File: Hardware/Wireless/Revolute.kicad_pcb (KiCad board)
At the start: 4 copper layers, 20 x 20 mm, 54 parts, among them Q1 AO3407, U1 BQ27441-G1, U2 nrf52833_qfn40, U3 AS5600, U4 AP2112K-3.3, U5 BQ24075RGT, U7 MAX16054, X1 32.768 kHz, X2 32MHZ

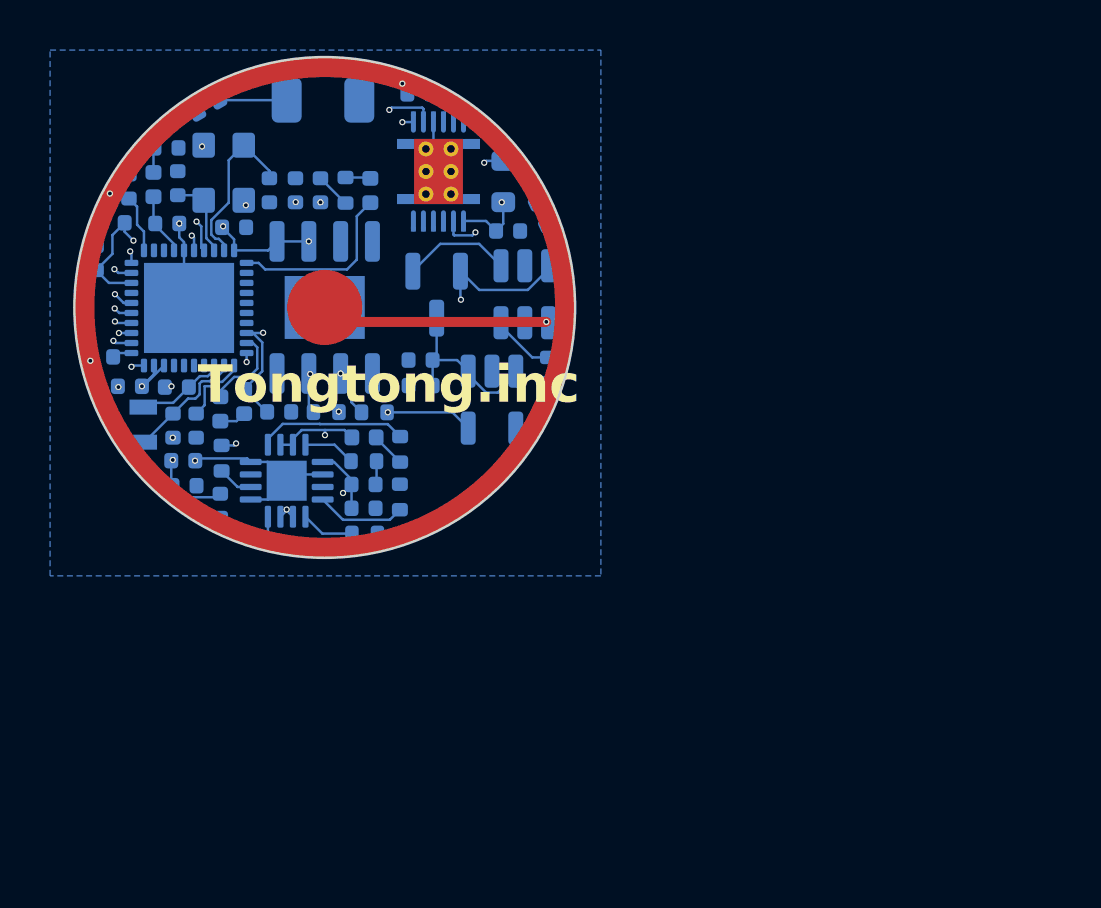
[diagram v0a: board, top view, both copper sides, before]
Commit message: worked on wireless
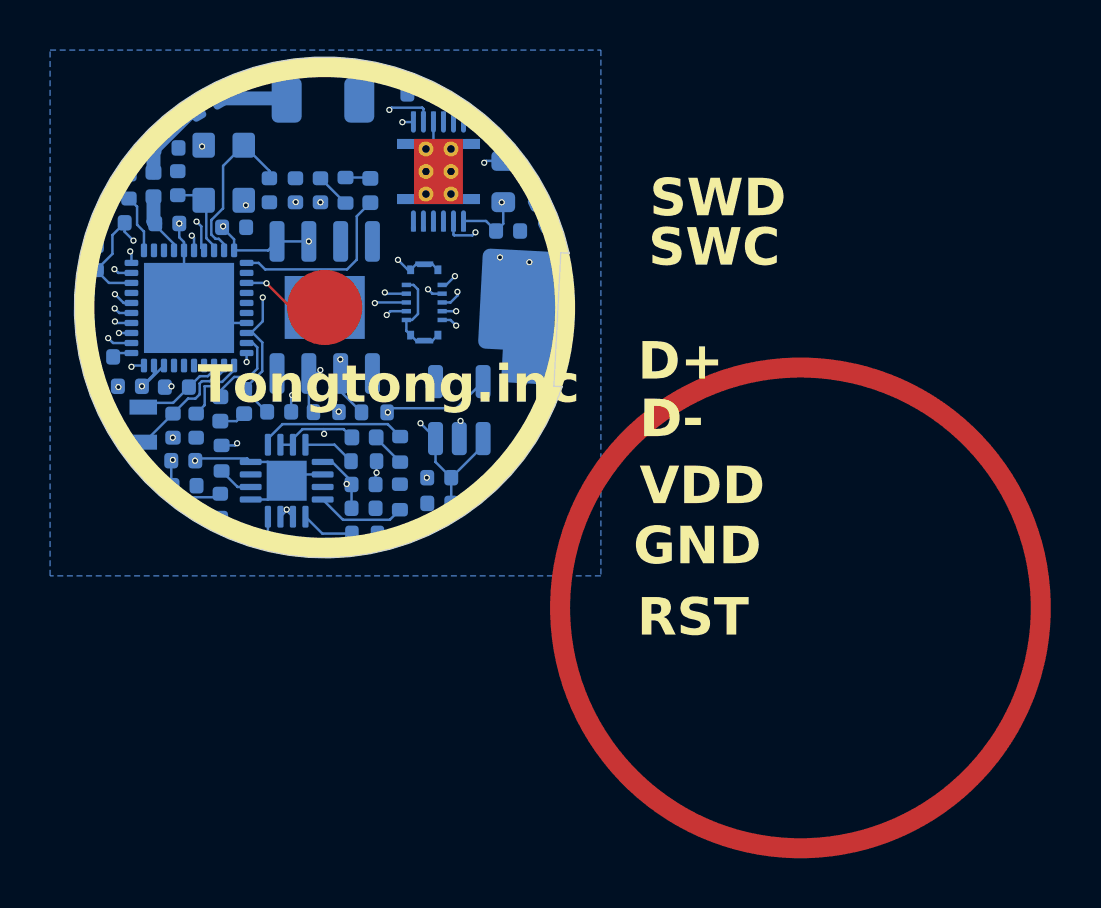
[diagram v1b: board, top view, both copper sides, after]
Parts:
- removed the ? at (171.0, 95.0)
- removed Q1: AO3407, Package_TO_SOT_SMD:SOT-23
- removed R10: 5.1K, Resistor_SMD:R_0402_1005Metric
- removed U7: MAX16054, Package_TO_SOT_SMD:SOT-23-6
- added ?: , , F.Cu at (179.1, 96.5)
- added ?: , , F.Cu at (178.7, 94.7)
- added U6: Button, Library:buttoncompliant, F.Cu at (171.0, 95.0)
- added U8: ~, Library:BK13C06-10DP, B.Cu at (175.0, 94.8)
- AE1: value ANT3216LL00R2400A -> Antenna
- moved C26 4.76 mm to (175.6, 102.8)
- moved C22 4.76 mm to (175.6, 101.8)
- moved U4 1.37 mm to (176.4, 99.1), turned to 90 degrees
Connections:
- C22 pad 1: vSYSTEM -> OUT
- C26 pad 1: vSYSTEM -> OUT
- U2 pad 33: unconnected-(U2-P0.28/AIN4-Pad33) -> Net-(U2-P0.28/AIN4)
- U4 pad 1: vSYSTEM -> OUT
- U4 pad 3: vSYSTEM -> OUT
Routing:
- net D+: track 0.76 -> 19.8 mm, vias 1 -> 2
- net D-: track 0.50 -> 17.6 mm, vias 1 -> 2
- net swd: track 0.74 -> 13.4 mm, vias 1 -> 2
- net swc: track 0.48 -> 13.0 mm, vias 1 -> 2
- net RESET: track 0.80 -> 13.1 mm, vias 1 -> 2
- net Net-(U7-IN): track 9.19 -> 0.00 mm, vias 1 -> 0
- net GND: track 20.3 -> 27.7 mm, vias 10 -> 24
- net vSYSTEM: track 7.14 -> 0.00 mm
- net OUT: track 22.9 -> 17.7 mm
- net Net-(Q1-G): track 4.33 -> 0.00 mm
- net Batteryin: track 6.56 -> 10.3 mm, vias 2 -> 4
- net VDD_nRF: track 18.6 -> 22.3 mm, vias 8 -> 10
- net Net-(U2-P0.28/AIN4): track 0.00 -> 3.53 mm, vias 0 -> 1
- net CLEAR: track 2.53 -> 0.00 mm
- net P0.15: track 28.6 -> 31.0 mm, vias 3 -> 4
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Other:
- board size 20 x 20 mm -> 19.8 x 20 mm
- board text added: "D+"
- board text added: "D-"
- board text added: "GND"
- board text added: "RST"
- board text added: "SWC"
- board text added: "SWD"
- board text added: "VDD"
